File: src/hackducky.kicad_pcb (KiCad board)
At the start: 4 copper layers, 49.8 x 25.2 mm, 65 parts, among them J1 USB_A, J2 Conn_02x02_Top_Bottom, J3 Micro_SD_Card, P2 USB_C_Plug, SW3 BOOT_SEL, SW4 BOOT_SEL, U1 W25Q16JVSS, U2 AMS1117-3.3, U4 RP2040, Y1 Crystal_GND24

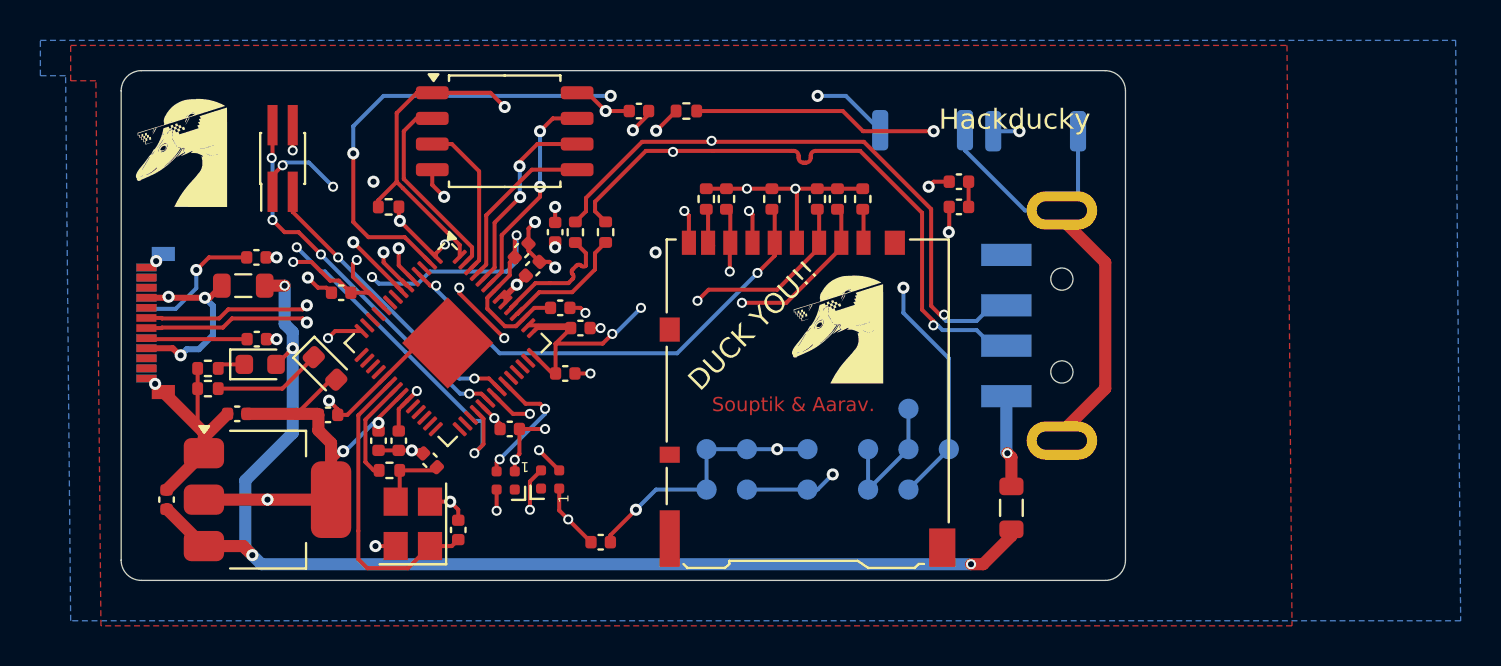
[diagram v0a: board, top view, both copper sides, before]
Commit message: f
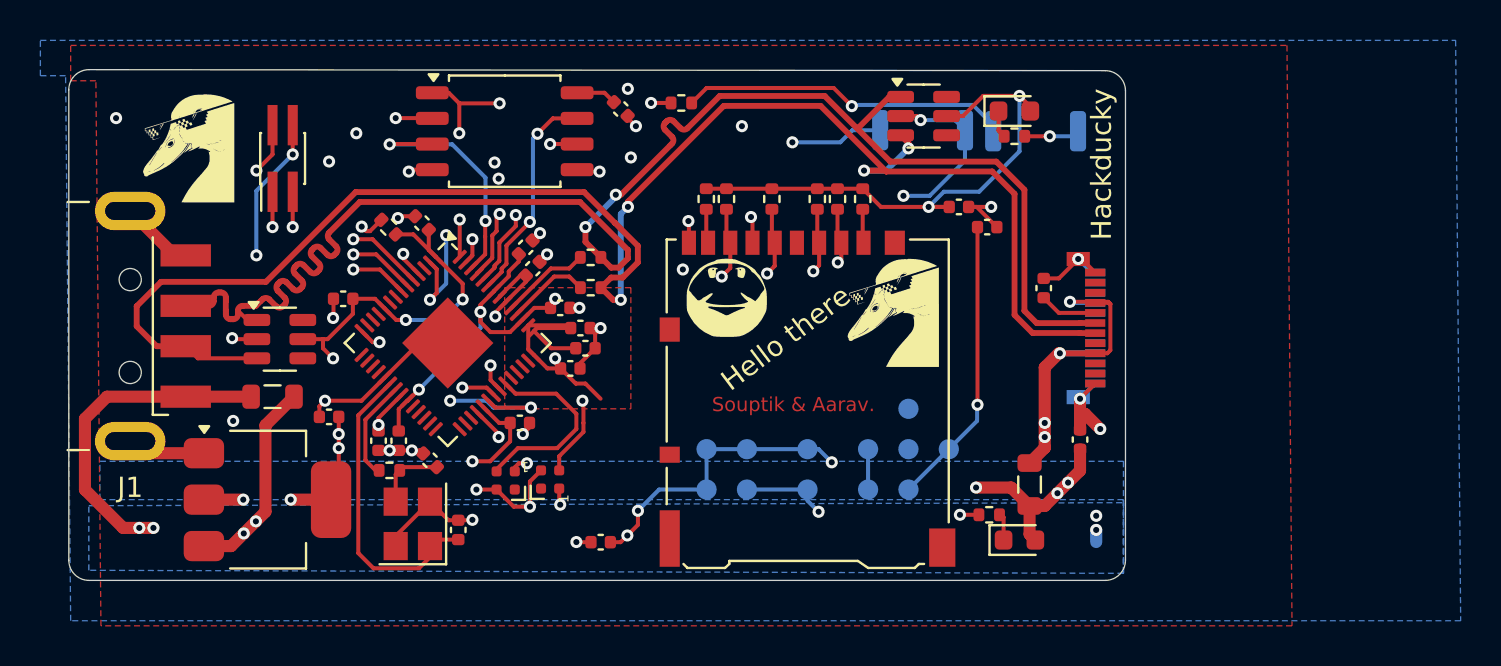
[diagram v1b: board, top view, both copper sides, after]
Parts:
- removed the G*** at (101.0, 87.5)
- removed R5: 5.1K, Capacitor_SMD:C_0402_1005Metric
- added G***: LOGO, LOGO, F.Cu at (92.5, 87.5)
- added G***: LOGO, LOGO, B.Cu at (101.0, 88.2)
- added U5: SRV05-4, Package_TO_SOT_SMD:SOT-23-6, F.Cu at (102.2, 78.5)
- added U6: SRV05-4, Package_TO_SOT_SMD:SOT-23-6, F.Cu at (70.4, 89.5)
- J1: moved to F.Cu
- moved J1 60.0 mm to (56.0, 88.9), turned to 180 degrees
- moved P2 47.1 mm to (110.8, 89.0), turned to -90 degrees
- moved C14 45.3 mm to (110.0, 94.5)
- moved R1 41.9 mm to (106.8, 79.5), turned to 0 degrees
- moved R2 39.4 mm to (105.5, 98.2)
- moved R4 39.1 mm to (108.2, 87.0), turned to 90 degrees
- moved D6 38.6 mm to (107.0, 99.5)
- moved D5 36.5 mm to (106.8, 78.2), turned to 0 degrees
- moved C17 13.2 mm to (85.5, 90.0)
- moved C10 6.62 mm to (77.4, 83.8), turned to 135 degrees
- moved FB1 5.69 mm to (70.0, 92.4)
- moved C15 4.55 mm to (72.8, 93.4)
- moved G*** 2.88 mm to (100.5, 85.9)
- moved R22 2.85 mm to (85.8, 87.0), turned to 0 degrees
- moved C25 2.65 mm to (105.4, 84.0)
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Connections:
- P2 pad B5: Net-(P2-VCONN) -> unconnected-(P2-VCONN-PadB5)
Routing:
- net +5V: track 86.1 -> 41.5 mm, vias 6 -> 8
- net VBUS: track 17.4 -> 40.7 mm, vias 4 -> 8
- net D-: track 64.1 -> 83.1 mm, vias 3 -> 4
- net +1V1: track 71.5 -> 54.4 mm, vias 6 -> 4
- net D+: track 63.1 -> 78.5 mm, vias 3 -> 2
- net Net-(P2-VCONN): track 6.57 -> 0.00 mm, vias 1 -> 0
- net GPIO22: track 19.1 -> 25.6 mm, vias 4 -> 3
- net +3V3: track 108.5 -> 102.1 mm, vias 20 -> 21
- net GPIO0: track 36.8 -> 30.8 mm, vias 3 -> 5
- net SD_CS: track 35.7 -> 30.5 mm
- net GND: track 83.0 -> 78.3 mm, vias 22 -> 28
- net GPIO23: track 22.9 -> 18.3 mm, vias 5 -> 2
- net QSPI_SD2: track 7.85 -> 12.4 mm, vias 0 -> 2
- net Net-(D5-K): track 5.38 -> 1.36 mm
- net GP25: track 6.58 -> 9.77 mm, vias 2 -> 0
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- added copper zone on B.Cu, net +3V3
- added copper zone on In2.Cu, net +5V
- added copper zone on B.Cu, net VBUS
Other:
- board size 49.8 x 25.2 mm -> 52.3 x 25.3 mm
- board text added: "Hello there"
- board text removed: "DUCK YOU!!"
